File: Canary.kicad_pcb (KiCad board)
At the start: 4 copper layers, 56 x 38 mm, 85 parts, among them J1 CONN_ARM_CM_JTAG_SWD_10, J2 20021311-00010T4LF, J3 USB4125-GF-A, J4 S2B-PH-SM4-TB, Q1 PMN30UNX, Q2 PMN42XPEAH, Q3 PMN30UNX, SW1 TL3301SPF160QJ, U1 BMD-300-A-R, U10 LP5907MFX-3.2, U11 MCP73831T-2ATI_OT, U12 MIC2288YD5, U2 DNP, U3 SHTC3, U4 SGP40, U5 MAX6071BAUT21T, U6 LMP91000, U7 DNP, U8 MCP6041T-I_OT, U9 RT6150AGQW, Y1 32.7680 kHz

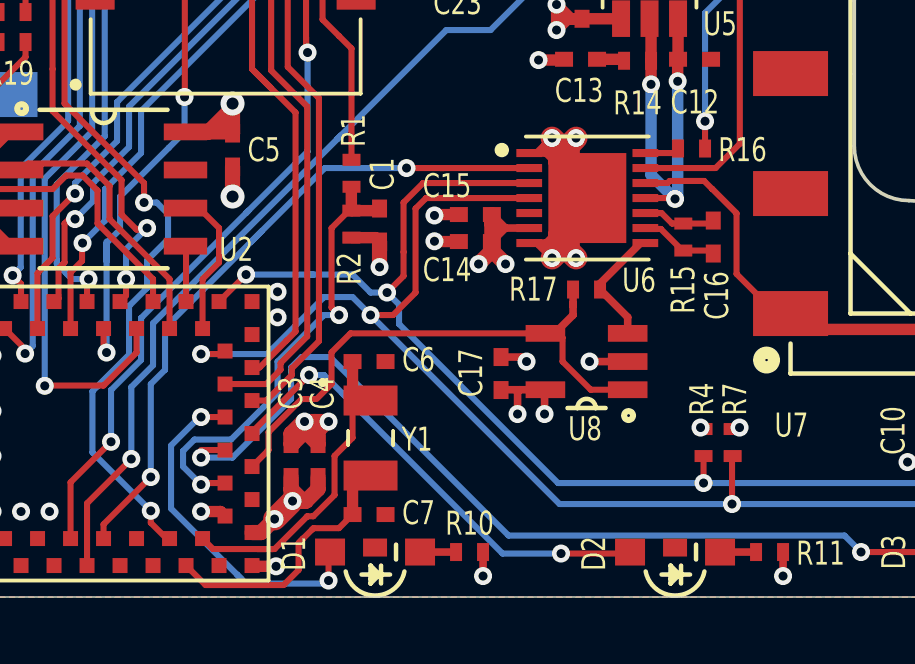
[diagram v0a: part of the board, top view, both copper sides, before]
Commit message: Change crystal again
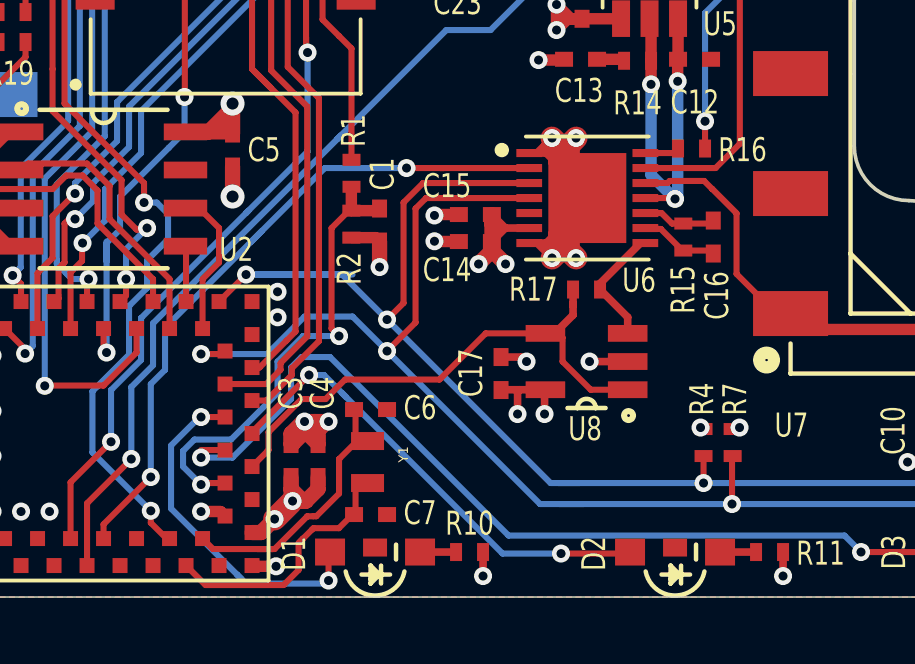
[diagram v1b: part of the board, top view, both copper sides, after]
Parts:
- Y1: footprint JetkovKiCADLib:FC135327680KAAC3 -> JetkovKiCADLib:ECS-327-9-12-C-TR
- moved C6 1.60 mm to (60.9, 79.8)
- moved Y1 0.81 mm to (60.8, 81.5)
- moved C7 0.05 mm to (60.9, 83.2)
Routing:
- net I2C_SCL: track 49.2 -> 54.0 mm
- net /XTAL2: track 11.8 -> 9.76 mm
- net I2C_SDA: track 51.9 -> 52.7 mm
- net LMP_VOUT_B: track 19.0 -> 18.4 mm
